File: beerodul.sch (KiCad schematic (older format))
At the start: 1 part

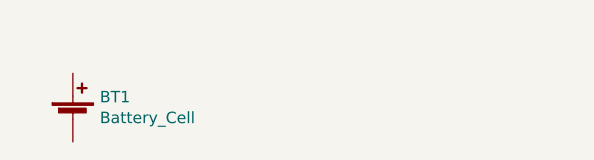
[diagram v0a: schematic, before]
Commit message: Work work
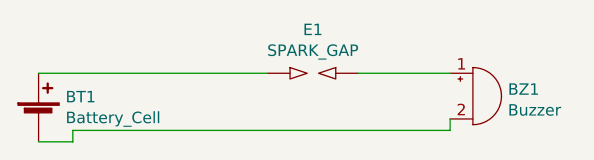
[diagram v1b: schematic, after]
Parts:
- added BZ1: Buzzer, Buzzer_Beeper:Buzzer_12x9.5RM7.6, symbol Device:Buzzer
- added E1: SPARK_GAP, symbol Device:SPARK_GAP
- BT1: footprint Battery:BatteryHolder_Keystone_103_1x20mm -> Battery:BatteryHolder_Keystone_106_1x20mm
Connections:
- net at BT1.1 (+): now also E1.1
- net at BT1.2 (-): now also BZ1.2 (+)
- new net: BZ1.1 (-), E1.2
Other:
- moved on the sheet: BT1
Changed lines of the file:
@@
 EESchema Schematic File Version 4
+LIBS:beerodul-cache
 EELAYER 26 0
 EELAYER END
@@
 L Device:Battery_Cell BT1
 U 1 1 5C2DFE60
-P 5300 3200
-F 0 "BT1" H 5418 3296 50  0000 L CNN
-F 1 "Battery_Cell" H 5418 3205 50  0000 L CNN
-F 2 "Battery:BatteryHolder_Keystone_103_1x20mm" V 5300 3260 50  0001 C CNN
-F 3 "~" V 5300 3260 50  0001 C CNN
-	1    5300 3200
+P 5150 3200
+F 0 "BT1" H 5268 3296 50  0000 L CNN
+F 1 "Battery_Cell" H 5268 3205 50  0000 L CNN
+F 2 "Battery:BatteryHolder_Keystone_106_1x20mm" V 5150 3260 50  0001 C CNN
+F 3 "~" V 5150 3260 50  0001 C CNN
+	1    5150 3200
 	1    0    0    -1
 $EndComp
+$Comp
+L Device:SPARK_GAP E1
+U 1 1 5C476CAB
+P 6350 3000
+F 0 "E1" H 6350 3190 50  0000 C CNN
+F 1 "SPARK_GAP" H 6350 3099 50  0000 C CNN
+F 2 "" H 6350 2930 50  0001 C CNN
+F 3 "~" V 6350 3000 50  0001 C CNN
+	1    6350 3000
+	1    0    0    -1
+$EndComp
+$Comp
+L Device:Buzzer BZ1
+U 1 1 5C476DE6
+P 7050 3100
+F 0 "BZ1" H 7203 3129 50  0000 L CNN
+F 1 "Buzzer" H 7203 3038 50  0000 L CNN
+F 2 "Buzzer_Beeper:Buzzer_12x9.5RM7.6" V 7025 3200 50  0001 C CNN
+F 3 "~" V 7025 3200 50  0001 C CNN
+	1    7050 3100
+	1    0    0    -1
+$EndComp
+Wire Wire Line
+	5150 3000 6150 3000
+Wire Wire Line
+	6950 3250 6950 3200
+Wire Wire Line
+	5300 3250 6950 3250
+Wire Wire Line
+	5300 3250 5300 3300
+Wire Wire Line
+	6550 3000 6950 3000
+Wire Wire Line
+	5150 3300 5300 3300
 $EndSCHEMATC
